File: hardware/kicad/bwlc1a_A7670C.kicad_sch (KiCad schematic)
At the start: 57 parts, among them J3 Nano SIM, J5 RSP-122811-02, Q1 NPN, Q2 NPN, Q5 NPN, Q6 NPN, U2 A7670C_24x24mm, U5 MIC29302WU

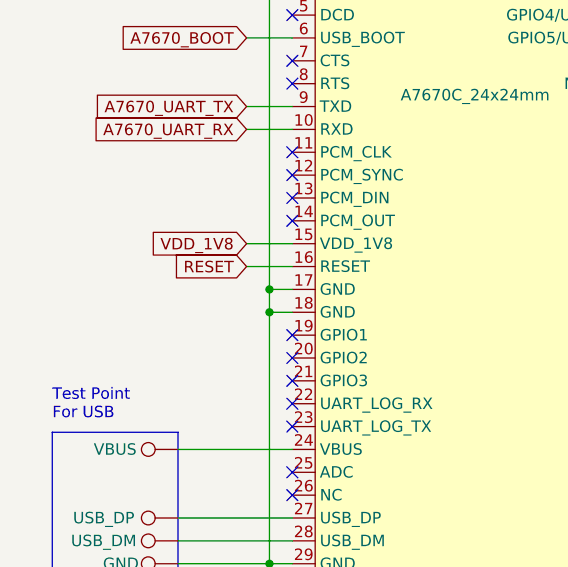
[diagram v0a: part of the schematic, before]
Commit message: Update on PCB Layout
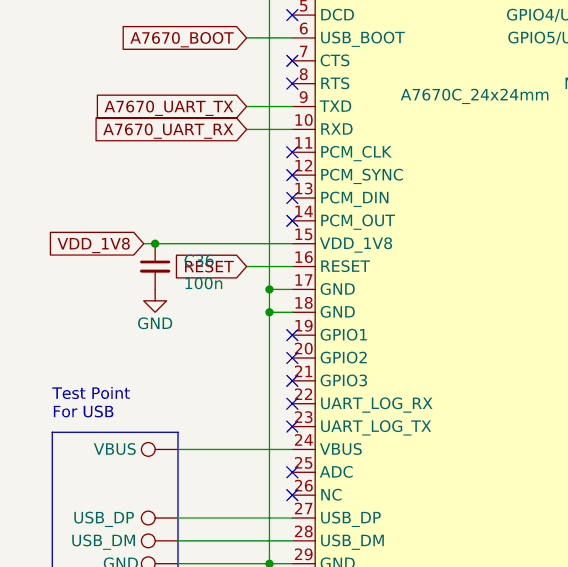
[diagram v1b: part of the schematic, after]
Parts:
- added C36: 100n, Capacitor_SMD:C_0402_1005Metric, symbol Device:C_Small
- C20, C21, C23: footprint Capacitor_SMD:C_0402_1005Metric -> Capacitor_SMD:C_0603_1608Metric
- C25: footprint Capacitor_SMD:C_0402_1005Metric -> Capacitor_SMD:C_0805_2012Metric
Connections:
- net GND: now also C36.2
- net VDD_1V8: now also C36.1
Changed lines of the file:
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@@
   (junction (at 139.065 107.442) (diameter 0) (color 0 0 0 0)
   )
+  (junction (at 27.305 112.395) (diameter 0) (color 0 0 0 0)
+  )
   (junction (at 40.005 173.355) (diameter 0) (color 0 0 0 0)
   )
@@
     (stroke (width 0) (type default))
   )
-  (wire (pts (xy 37.465 112.395) (xy 42.545 112.395))
+  (wire (pts (xy 26.035 112.395) (xy 27.305 112.395))
     (stroke (width 0) (type default))
   )
@@
     (stroke (width 0) (type default))
   )
+  (wire (pts (xy 27.305 112.395) (xy 42.545 112.395))
+    (stroke (width 0) (type default))
+  )
   (wire (pts (xy 87.63 109.855) (xy 87.63 99.695))
     (stroke (width 0) (type default))
@@
     )
   )
-  (global_label "VDD_1V8" (shape input) (at 37.465 112.395 180) (fields_autoplaced)
+  (global_label "VDD_1V8" (shape input) (at 26.035 112.395 180) (fields_autoplaced)
     (effects (font (size 1.27 1.27)) (justify right))
-    (property "Intersheetrefs" "${INTERSHEET_REFS}" (at 26.4554 112.395 0)
+    (property "Intersheetrefs" "${INTERSHEET_REFS}" (at 15.0254 112.395 0)
       (effects (font (size 1.27 1.27)) (justify right) hide)
     )
@@
       (effects (font (size 1.27 1.27)) (justify left))
     )
-    (property "Footprint" "Capacitor_SMD:C_0402_1005Metric" (at 140.97 79.375 0)
+    (property "Footprint" "Capacitor_SMD:C_0603_1608Metric" (at 140.97 79.375 0)
       (effects (font (size 1.27 1.27)) hide)
     )
@@
       (effects (font (size 1.27 1.27)) (justify left))
     )
-    (property "Footprint" "Capacitor_SMD:C_0402_1005Metric" (at 48.26 36.195 0)
+    (property "Footprint" "Capacitor_SMD:C_0603_1608Metric" (at 48.26 36.195 0)
       (effects (font (size 1.27 1.27)) hide)
     )
@@
       (effects (font (size 1.27 1.27)) (justify left))
     )
-    (property "Footprint" "Capacitor_SMD:C_0402_1005Metric" (at 121.285 36.195 0)
+    (property "Footprint" "Capacitor_SMD:C_0805_2012Metric" (at 121.285 36.195 0)
       (effects (font (size 1.27 1.27)) hide)
     )
@@
       (effects (font (size 1.27 1.27)) (justify left))
     )
-    (property "Footprint" "Capacitor_SMD:C_0402_1005Metric" (at 150.495 79.375 0)
+    (property "Footprint" "Capacitor_SMD:C_0603_1608Metric" (at 150.495 79.375 0)
       (effects (font (size 1.27 1.27)) hide)
     )
@@
     )
   )
+  (symbol (lib_id "Device:C_Small") (at 27.305 114.935 0) (unit 1)
+    (in_bom yes) (on_board yes) (dnp no) (fields_autoplaced)
+    (property "Reference" "C36" (at 30.48 114.3063 0)
+      (effects (font (size 1.27 1.27)) (justify left))
+    )
+    (property "Value" "100n" (at 30.48 116.8463 0)
+      (effects (font (size 1.27 1.27)) (justify left))
+    )
+    (property "Footprint" "Capacitor_SMD:C_0402_1005Metric" (at 27.305 114.935 0)
+      (effects (font (size 1.27 1.27)) hide)
+    )
+    (property "Datasheet" "~" (at 27.305 114.935 0)
+      (effects (font (size 1.27 1.27)) hide)
+    )
+    (pin "1")
+    (pin "2")
+    (instances
+      (project "bwlc1a"
+        (path "/388039b1-99cc-430f-bd4a-010573fde798"
+          (reference "C36") (unit 1)
+        )
+        (path "/388039b1-99cc-430f-bd4a-010573fde798/d0b0fe7e-ffcb-4a20-b7b5-70f0caeaf6a1"
+          (reference "C38") (unit 1)
+        )
+      )
+    )
+  )
   (symbol (lib_id "power:GND") (at 115.57 116.84 0) (unit 1)
     (in_bom yes) (on_board yes) (dnp no)
@@
         )
       )
+    )
+  )
+  (symbol (lib_id "power:GND") (at 27.305 117.475 0) (unit 1)
+    (in_bom yes) (on_board yes) (dnp no)
+    (property "Reference" "#PWR063" (at 27.305 123.825 0)
+      (effects (font (size 1.27 1.27)) hide)
+    )
+    (property "Value" "GND" (at 27.305 121.285 0)
+      (effects (font (size 1.27 1.27)))
+    )
+    (property "Footprint" "" (at 27.305 117.475 0)
+      (effects (font (size 1.27 1.27)) hide)
+    )
+    (property "Datasheet" "" (at 27.305 117.475 0)
+      (effects (font (size 1.27 1.27)) hide)
+    )
+    (pin "1")
+    (instances
+      (project "bwlc1a"
+        (path "/388039b1-99cc-430f-bd4a-010573fde798"
+          (reference "#PWR063") (unit 1)
+        )
+        (path "/388039b1-99cc-430f-bd4a-010573fde798/d0b0fe7e-ffcb-4a20-b7b5-70f0caeaf6a1"
+          (reference "#PWR089") (unit 1)
+        )
+      )
